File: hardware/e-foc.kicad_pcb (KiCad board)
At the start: 4 copper layers, 89.4 x 66.9 mm, 186 parts, among them J1 Screw_Terminal_01x02, J2 Screw_Terminal_01x03, J3 Screw_Terminal_01x02, J4 Conn_01x05_Pin, J5 Conn_01x03, J6 Conn_02x12_Odd_Even, J7 Conn_02x06_Odd_Even, Q1 CSD88537ND, Q2 CSD88537ND, Q3 CSD88537ND, Q4 BC847, Q5 BC847, Q6 BC847, SW1 SW_DIP_x03, U1 LM5164DDA, U10 W25Q32JVSS, U2 LM317_SOT-223, U3 AMS1117-3.3, U4 FAN7888, U5 TLV9064, U6 TLV9062, U7 SN65HVD230, U8 74LVC14, U9 24LC04

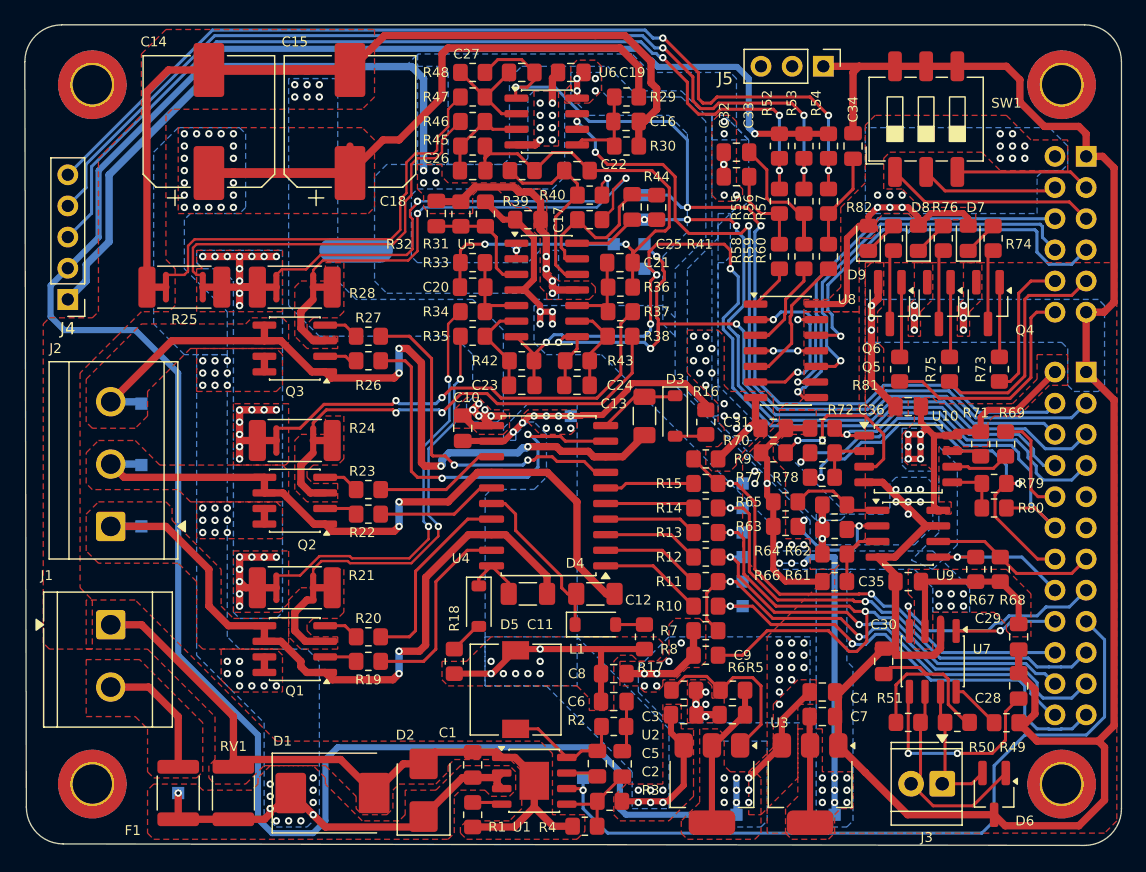
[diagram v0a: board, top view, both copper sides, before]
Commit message: updates
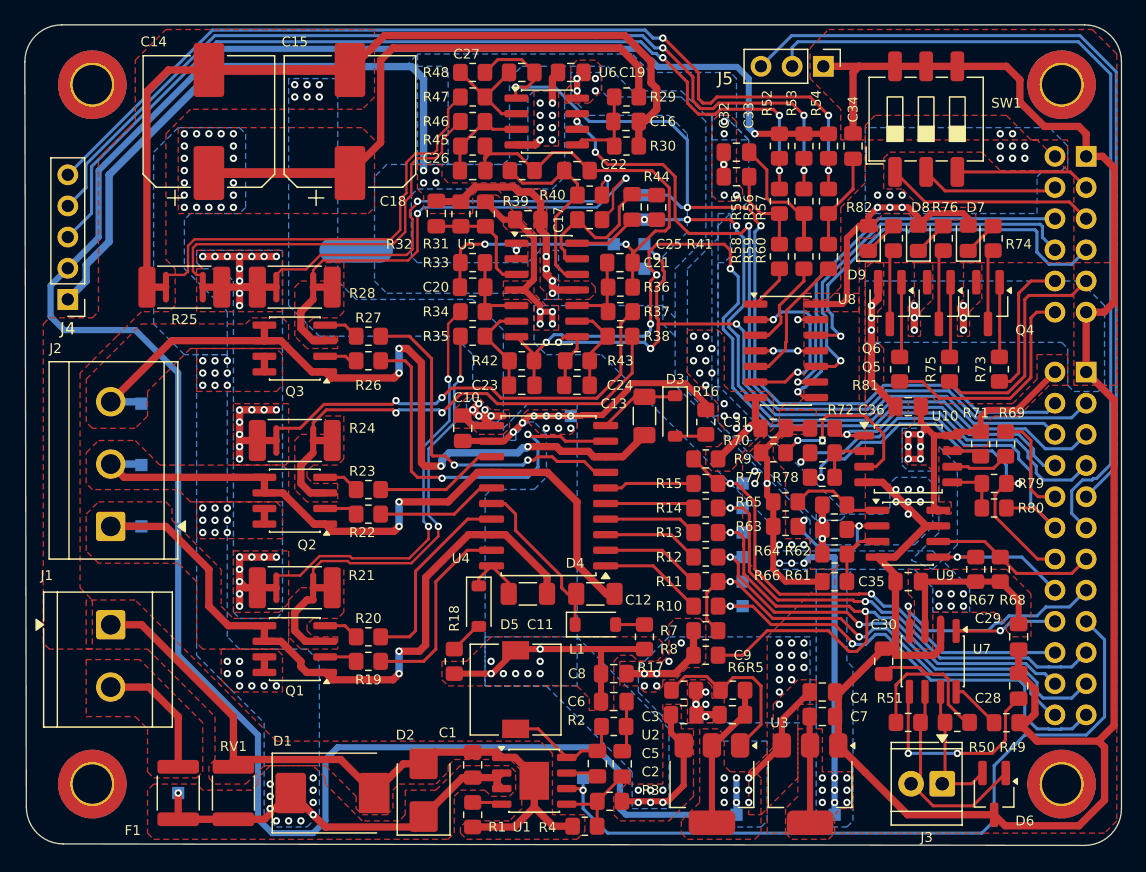
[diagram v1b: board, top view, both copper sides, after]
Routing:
- net Net-(J5-Pin_2): track 0.00 -> 68.2 mm
- net Net-(J5-Pin_3): track 0.00 -> 66.9 mm
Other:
- copper layers 4 -> 2
